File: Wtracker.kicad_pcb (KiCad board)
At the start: 2 copper layers, 32 parts, among them IC1 RFX2401C, U1 GPS, U2 ATGM336H-5N31, U4 NRF52840-QIAA-R, X1 NX2016SA-32MHZ-STD-CZS-5

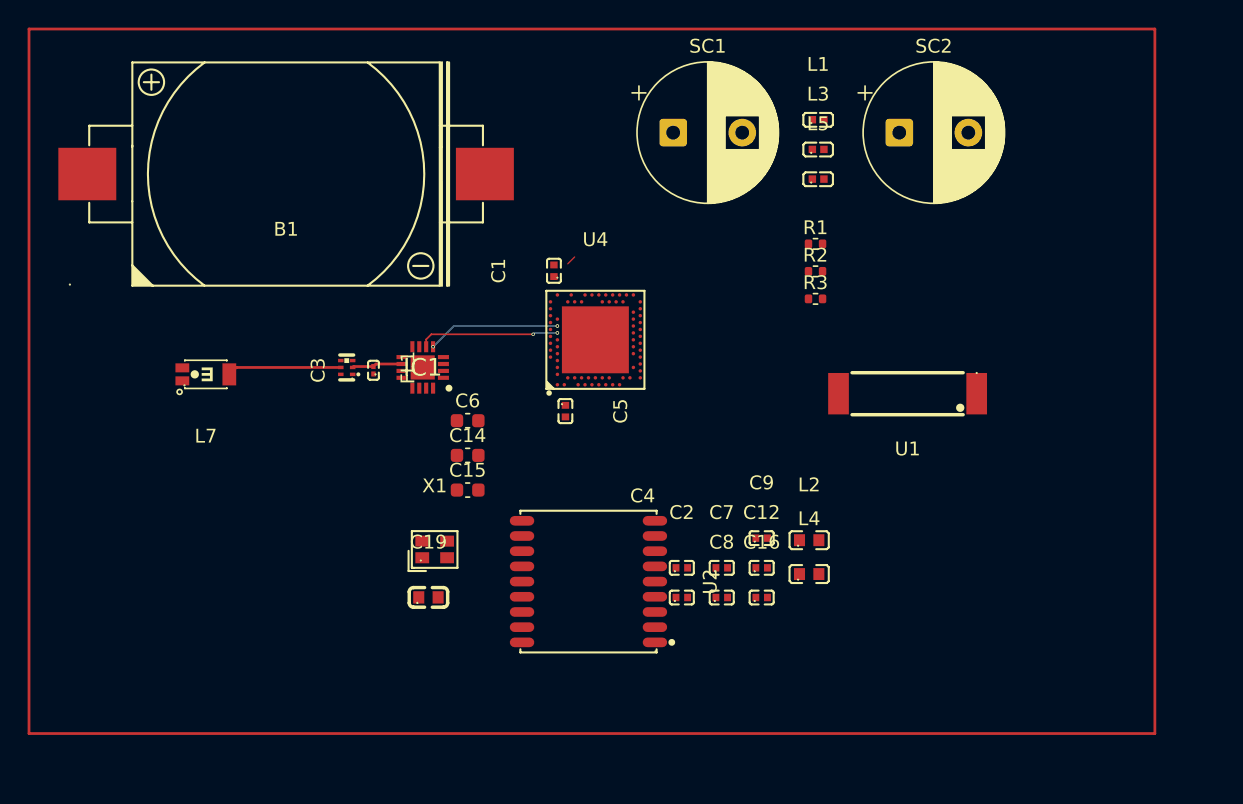
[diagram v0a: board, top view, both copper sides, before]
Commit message: updated pcb and schematic and BOM
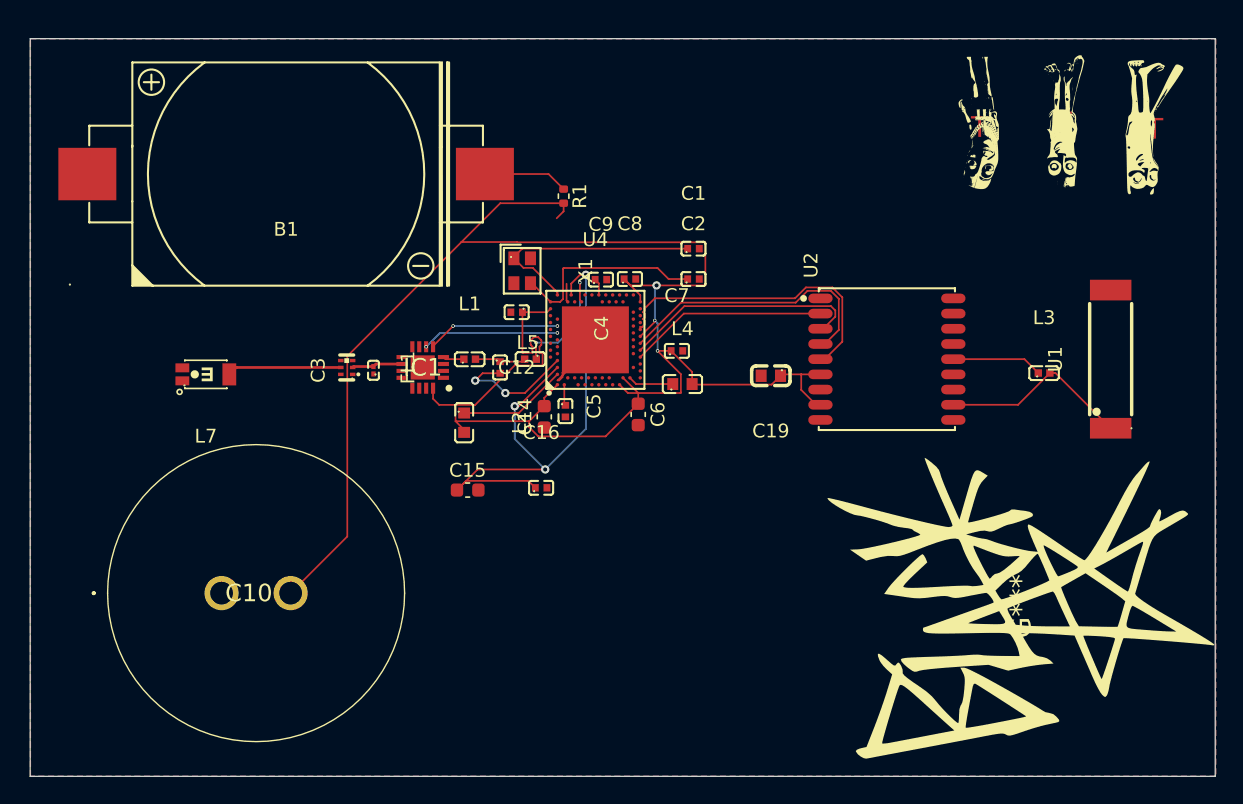
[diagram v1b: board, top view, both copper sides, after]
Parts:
- removed R2, R3: 100Ω, Resistor_SMD:R_0402_1005Metric
- removed SC1, SC2: 3F,2.7V, Capacitor_THT:CP_Radial_D10.0mm_P5.00mm
- added C10: KR-5R5C155-R, KR-5R5C155-R:KR5R5C155R, F.Cu at (115.4, 103.3)
- added G***: LOGO, LOGO, F.Cu at (173.3, 104.3)
- added T: LOGO, LOGO, F.Cu at (176.4, 69.3)
- added T: LOGO, LOGO, F.Cu at (170.3, 69.5)
- added T: LOGO, LOGO, F.Cu at (183.0, 69.7)
- FL1: value H.Filter -> 2450LP14A100T
- moved L1 30.6 mm to (133.4, 86.4)
- moved C19 29.5 mm to (155.2, 87.6), turned to 180 degrees
- moved U2 26.9 mm to (163.6, 86.4), turned to 90 degrees
- moved L2 26.4 mm to (133.0, 91.0), turned to -90 degrees
- moved C12 25.6 mm to (136.8, 83.0), turned to 180 degrees
- moved L5 24.6 mm to (137.8, 86.4), turned to 180 degrees
- moved C8 24.0 mm to (145.0, 80.6)
- moved L3 23.0 mm to (175.0, 87.4)
- moved C9 22.0 mm to (142.9, 80.6)
- moved C4 21.2 mm to (135.6, 87.0), turned to -90 degrees
- moved X1 21.1 mm to (137.2, 80.0), turned to -90 degrees
- moved C2 20.9 mm to (149.6, 80.6)
- moved R1 18.6 mm to (140.2, 74.6), turned to -90 degrees
- moved C16 17.8 mm to (138.6, 95.7)
- moved L4 16.5 mm to (148.8, 88.2)
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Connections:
- B1 pad 2: /VBATT -> /BATT_RAW
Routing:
- net /VBATT: track 0.00 -> 144.0 mm, vias 0 -> 3
- net /DEC4: track 0.00 -> 40.4 mm, vias 0 -> 3
- net /On/Off: track 0.00 -> 22.5 mm
- net /1PPS: track 0.00 -> 20.2 mm
- net /GPS_RX: track 0.00 -> 17.5 mm
- net /XC1: track 0.00 -> 17.3 mm
- net /XC2: track 0.00 -> 14.6 mm
- net /GPS_TX: track 0.00 -> 14.3 mm
- net /RF_signal_G: track 0.00 -> 14.0 mm
- net GND: track 0.00 -> 9.31 mm, vias 0 -> 2
- net /ANT: track 0.00 -> 9.27 mm, vias 0 -> 2
- net unconnected-(U4-EP-Pad0): track 0.00 -> 8.21 mm
- net /DCC: track 0.00 -> 7.91 mm
- net /VCC_RF: track 0.00 -> 6.56 mm
- net /BATT_RAW: track 0.00 -> 6.15 mm
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- added copper zone on B.Cu, net GND
- added copper zone on F.Cu, net GND
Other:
- board outline added: 85.8 x 53.4 mm
- board text added: "3.9nH"
